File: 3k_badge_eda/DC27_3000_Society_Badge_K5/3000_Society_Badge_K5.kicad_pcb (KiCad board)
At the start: 2 copper layers, 195.2 x 165.9 mm, 28 parts, among them IC1 Trinket_M0

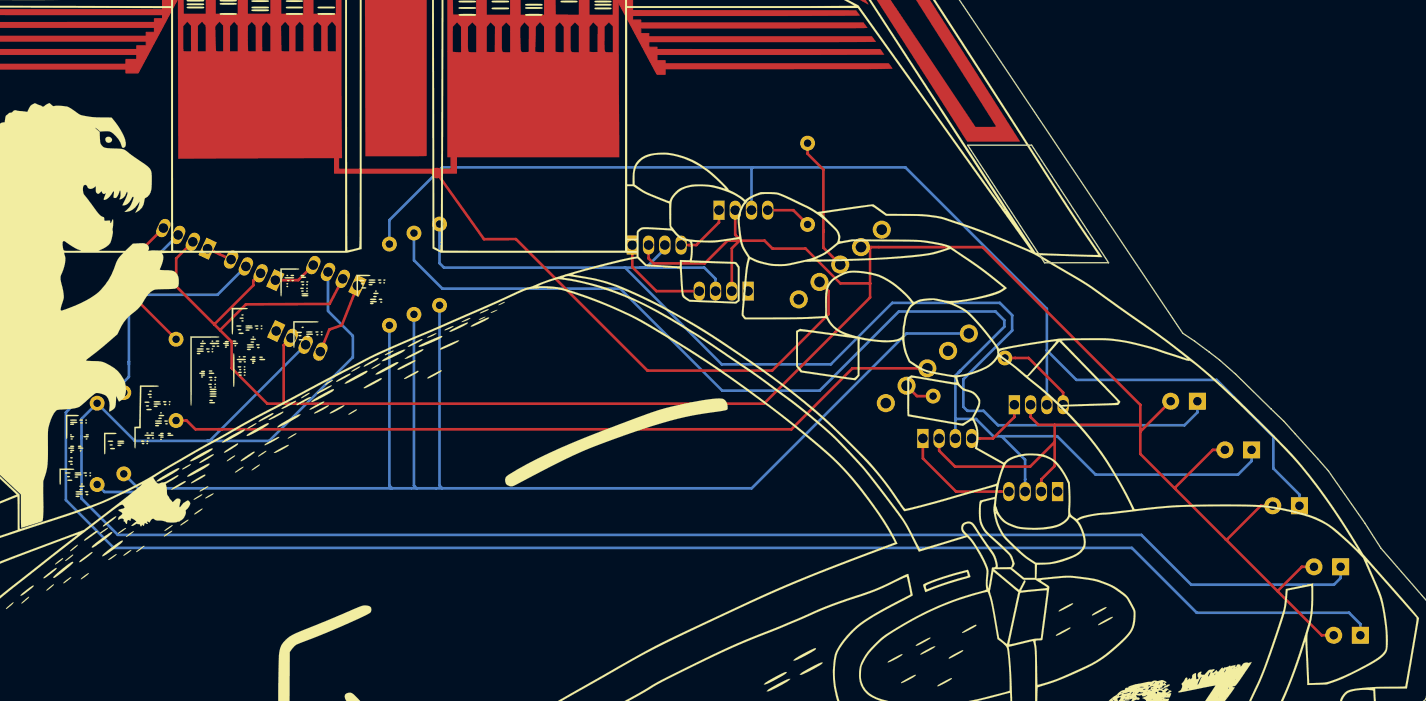
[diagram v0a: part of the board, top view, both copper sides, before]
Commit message: DC27_badge_redesign
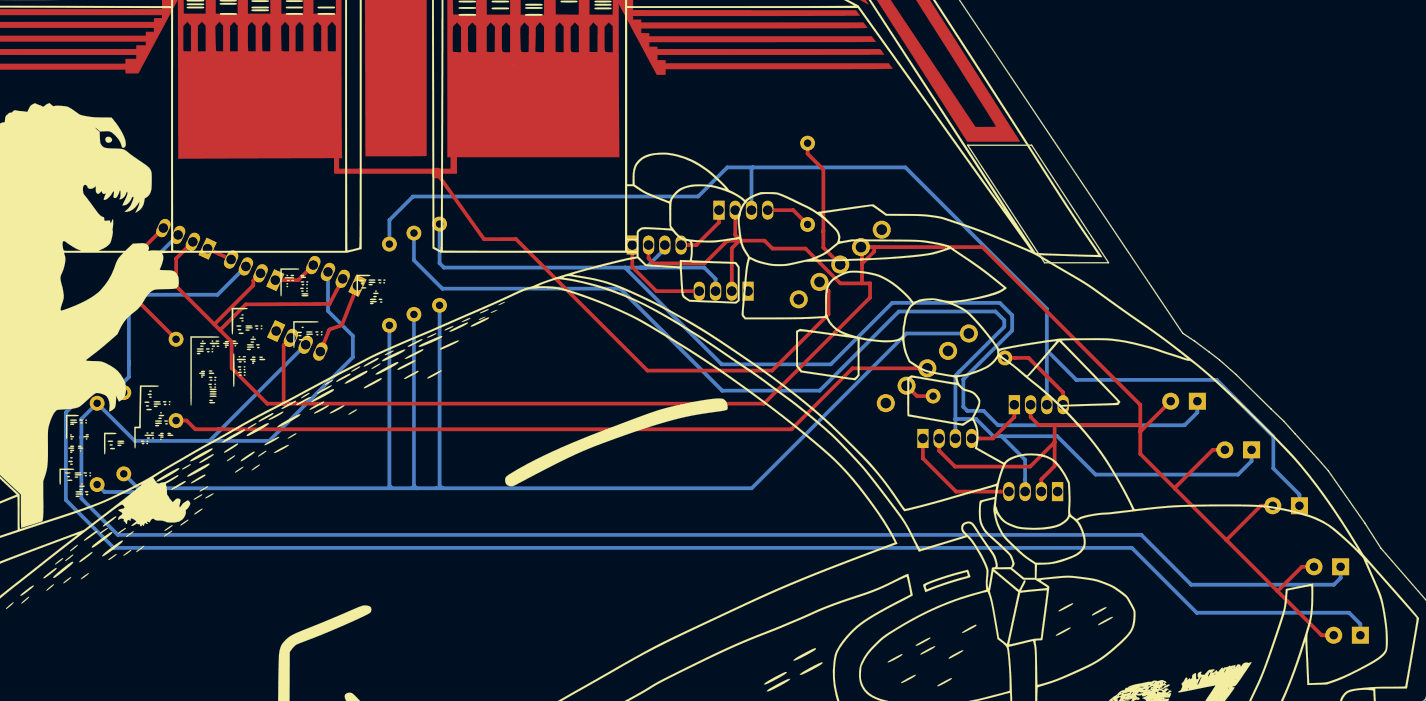
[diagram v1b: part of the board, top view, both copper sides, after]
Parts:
- removed the ? at (140.8, 36.4)
- added G***: HackFtW_Logo_Back_5000dpi, 3000_Society_Badge:HackFtW_Logo_Back_5000dpi, F.Cu at (106.8, 58.1)
- added G***: TheLabms_Logo_Back_1000dpi, 3000_Society_Badge:TheLabms_Logo_Back_1000dpi, F.Cu at (106.3, 69.6)
- added G***: DHA_Logo_Back_1500dpi, 3000_Society_Badge:DHA_Logo_Back_1500dpi, F.Cu at (128.1, 49.6)
- added G***: DC214_Logo_Back_4000dpi, 3000_Society_Badge:DC214_Logo_Back_4000dpi, F.Cu at (155.4, 48.0)
- added G***: BSidesDFW_Logo_Back_3500dpi, 3000_Society_Badge:BSidesDFW_Logo_Back_3500dpi, F.Cu at (145.0, 67.8)
- added G***: 3000_Society_Logo_Back_2500dpi, 3000_Society_Badge:3000_Society_Logo_Back_2500dpi, F.Cu at (176.9, 60.0)
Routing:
- net Net-(C1-Pad2): track 259.3 -> 261.2 mm
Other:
- net class Default: trace_width 0.25 -> 0.35
- board text added: "Altbier and Chill ---------- @alt_bier @r3x3r @t3hub3rk1tten"
- board text added: "Badge by @alt_bier and team Altbier and Chill"
- board text added: "Blade Runner"
- board text added: "Dedicated to:"
- board text added: "Godzilla vs."
- board text added: "https://3kbadge.altbier.us/"
- board text removed: "Badge Design by @alt_bier https://3kbadge.altbier.us/"
- board text removed: "DFW Hackers"
- board text removed: "Godzilla vs. Blade Runner"
- board text removed: "Presents"
- board text removed: "Supporting"
- board text removed: "https://3000society.com/"
